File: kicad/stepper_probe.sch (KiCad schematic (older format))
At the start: 50 parts, among them J1 Conn_01x04_Male, J2 Conn_01x04_Male, J3 BAT, J4 Serial Port, J5 SWD, J6 BAT, J7 Conn_01x01_Female, J8 Conn_01x01_Female, M1 Motor, SW1 SW_Push, U1 TMCS1108A4BQDT, U2 TMCS1108A4BQDT, U3 MDBT42Q-512KV2, U4 K7803MT-500R4, U5 M24C02-FMN, Y1 32.768Khz

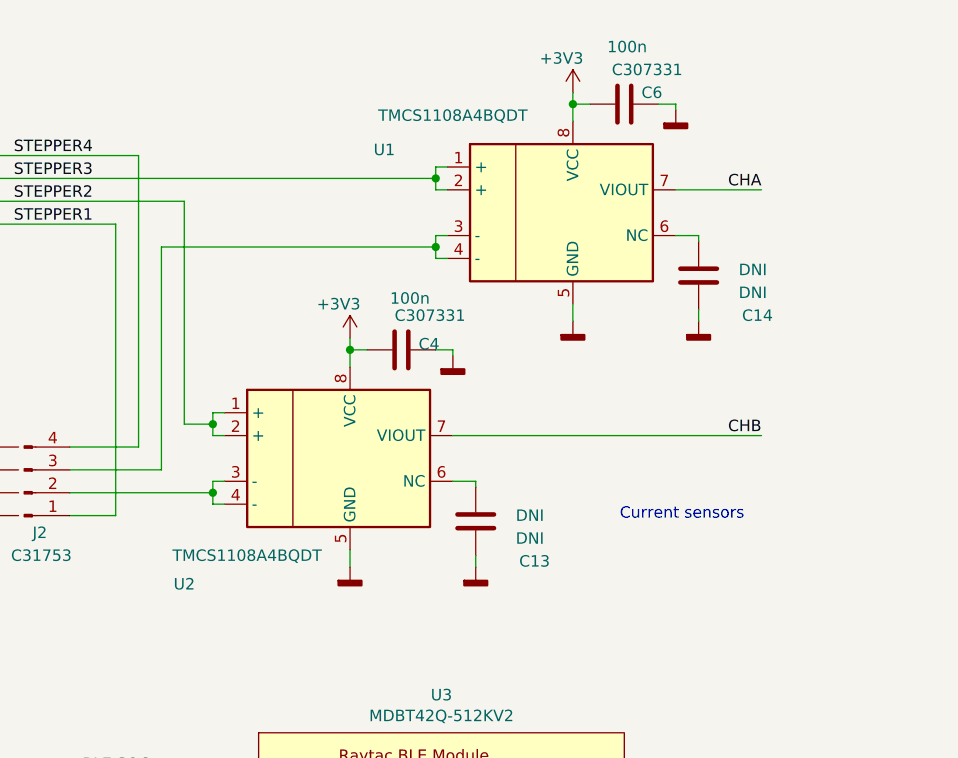
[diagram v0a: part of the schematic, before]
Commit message: .
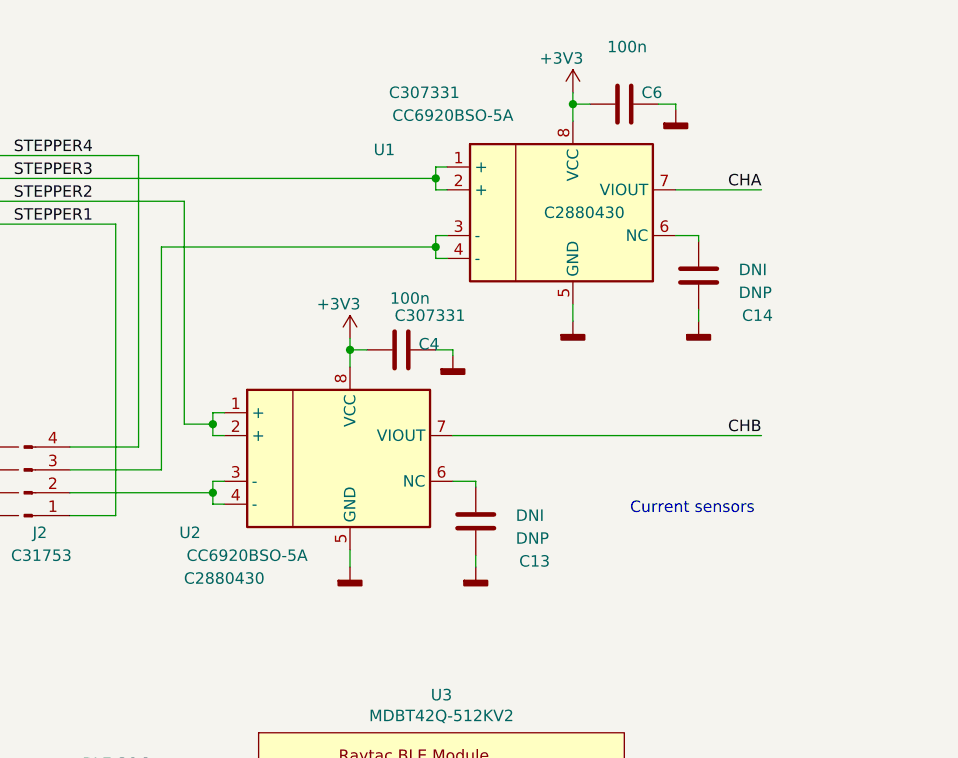
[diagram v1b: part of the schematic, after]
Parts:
- C13, C14: LCSC DNI -> DNP
- J7, J8, M1, R11, R12: LCSC (none) -> DNP
- U1, U2: value TMCS1108A4BQDT -> CC6920BSO-5A; LCSC (none) -> C2880430
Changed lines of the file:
@@
 F 2 "stepper_probe:connector_4pins_horizontal" H 950 1650 50  0001 C CNN
 F 3 "~" H 950 1650 50  0001 C CNN
+F 4 "" H 950 1650 50  0001 C CNN "LCSC"
 	1    950  1650
 	1    0    0    1
@@
 F 3 "~" H 1275 2925 50  0001 C CNN
 F 4 "C31753" H 1350 3200 50  0000 C CNN "LCSC Part Number"
+F 5 "" H 1275 2925 50  0001 C CNN "LCSC"
 	1    1275 2925
 	1    0    0    1
@@
 P 3725 1700
 F 0 "U1" H 2850 1975 50  0000 C CNN
-F 1 "TMCS1108A4BQDT" H 3150 2125 50  0000 C CNN
+F 1 "CC6920BSO-5A" H 3150 2125 50  0000 C CNN
 F 2 "Package_SO:SOIC-8_3.9x4.9mm_P1.27mm" H 4125 1650 50  0001 L CIN
 F 3 "" H 3725 1700 50  0001 C CNN
+F 4 "C2880430" H 3725 1700 50  0000 C CNN "LCSC"
 	1    3725 1700
 	1    0    0    -1
@@
 F 2 "stepper_probe:Empty" H 1010 3115 50  0001 C CNN
 F 3 "" H 1010 3115 50  0001 C CNN
+F 4 "DNP" H 1000 3025 50  0001 C CNN "LCSC"
 	1    1000 3025
 	0    -1   -1   0
@@
 	1    0    0    -1
 $EndComp
-Text Notes 4425 3050 2    50   ~ 0
-Current sensors
 $Comp
 L Connector:Conn_01x02_Male J3
@@
 F 2 "stepper_probe:PinHeader_1x02_P2.54mm_Vertical" H 8225 1025 50  0001 C CNN
 F 3 "~" H 8225 1025 50  0001 C CNN
+F 4 "" H 8225 1025 50  0001 C CNN "LCSC"
 	1    8225 1025
 	-1   0    0    -1
@@
 F 2 "stepper_probe:C_0402_1005Metric_Pad0.74x0.62mm_HandSolder" H 3938 1075 50  0001 C CNN
 F 3 "~" H 3900 1225 50  0001 C CNN
-F 4 "C307331" V 3750 1325 50  0000 C CNN "LCSC"
+F 4 "C307331" V 3850 350 50  0000 C CNN "LCSC"
 	1    3900 1225
 	0    1    1    0
@@
 F 2 "stepper_probe:PinHeader_1x04_P2.54mm_Vertical" H 10375 3675 50  0001 C CNN
 F 3 "~" H 10375 3675 50  0001 C CNN
+F 4 "" H 10375 3675 50  0001 C CNN "LCSC"
 	1    10375 3675
 	-1   0    0    -1
@@
 F 2 "stepper_probe:PinHeader_1x02_P2.54mm_Vertical" H 5250 4625 50  0001 C CNN
 F 3 "~" H 5250 4625 50  0001 C CNN
+F 4 "" H 5250 4625 50  0001 C CNN "LCSC"
 	1    5250 4625
 	-1   0    0    -1
@@
 F 2 "stepper_probe:C_0402_1005Metric_Pad0.74x0.62mm_HandSolder" H 3288 2900 50  0001 C CNN
 F 3 "~" H 3250 3050 50  0001 C CNN
-F 4 "DNI" H 3075 3125 50  0000 R CNN "LCSC"
+F 4 "DNP" H 3075 3125 50  0000 R CNN "LCSC"
 	1    3250 3050
 	-1   0    0    1
@@
 U 1 1 627AA0D1
 P 2750 2775
-F 0 "U2" H 1975 2225 50  0000 C CNN
-F 1 "TMCS1108A4BQDT" H 2250 2350 50  0000 C CNN
+F 0 "U2" H 2000 2450 50  0000 C CNN
+F 1 "CC6920BSO-5A" H 2250 2350 50  0000 C CNN
 F 2 "Package_SO:SOIC-8_3.9x4.9mm_P1.27mm" H 3150 2725 50  0001 L CIN
 F 3 "" H 2750 2775 50  0001 C CNN
+F 4 "C2880430" H 2150 2250 50  0000 C CNN "LCSC"
 	1    2750 2775
 	1    0    0    -1
@@
 F 2 "stepper_probe:C_0402_1005Metric_Pad0.74x0.62mm_HandSolder" H 4263 1825 50  0001 C CNN
 F 3 "~" H 4225 1975 50  0001 C CNN
-F 4 "DNI" H 4050 2050 50  0000 R CNN "LCSC"
+F 4 "DNP" H 4050 2050 50  0000 R CNN "LCSC"
 	1    4225 1975
 	-1   0    0    1
@@
 F 2 "stepper_probe:BAT_PLUS_PAD" H 6650 3550 50  0001 C CNN
 F 3 "~" H 6650 3550 50  0001 C CNN
+F 4 "DNP" H 6650 3550 50  0001 C CNN "LCSC"
 	1    6650 3550
 	1    0    0    -1
@@
 F 2 "stepper_probe:BAT_MINUS_PAD" H 6650 3775 50  0001 C CNN
 F 3 "~" H 6650 3775 50  0001 C CNN
+F 4 "DNP" H 6650 3775 50  0001 C CNN "LCSC"
 	1    6650 3775
 	1    0    0    -1
@@
 F 2 "stepper_probe:R_0402_1005Metric_Pad0.72x0.64mm_HandSolder" H 4975 6800 50  0001 C CNN
 F 3 "~" H 4975 6800 50  0001 C CNN
+F 4 "DNP" H 4975 6800 50  0001 C CNN "LCSC"
 	1    4975 6800
 	0    -1   -1   0
@@
 F 2 "stepper_probe:R_0402_1005Metric_Pad0.72x0.64mm_HandSolder" H 4975 7150 50  0001 C CNN
 F 3 "~" H 4975 7150 50  0001 C CNN
+F 4 "DNP" H 4975 7150 50  0001 C CNN "LCSC"
 	1    4975 7150
 	0    -1   -1   0
@@
 Text Notes 6100 4200 0    50   ~ 0
 9V battery pads for zero \ncurrent calibration.
+Text Notes 3925 3025 0    50   ~ 0
+Current sensors
 $EndSCHEMATC
